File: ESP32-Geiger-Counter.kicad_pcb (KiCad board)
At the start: 2 copper layers, 137 x 104 mm, 85 parts, among them J1 2s1p Lipo Battery Pack (8.4V-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, J2 USB_C_Receptacle_USB2.0_16P, J5 Conn_01x07, Q1 STN1HNK60, Q3 2N7002, Q4 AO3401A, Q5 MMBT3904, SW1 SW_SPDT, SW2 RESET, SW3 BOOT, U1 BQ25886RGE, U2 AP63203WU, U3 ESP32-S3-WROOM-1, U4 UCC27517DBVR, U5 USBLC6-2SC6, U6 SBM-20 Geiger Mueller Tube

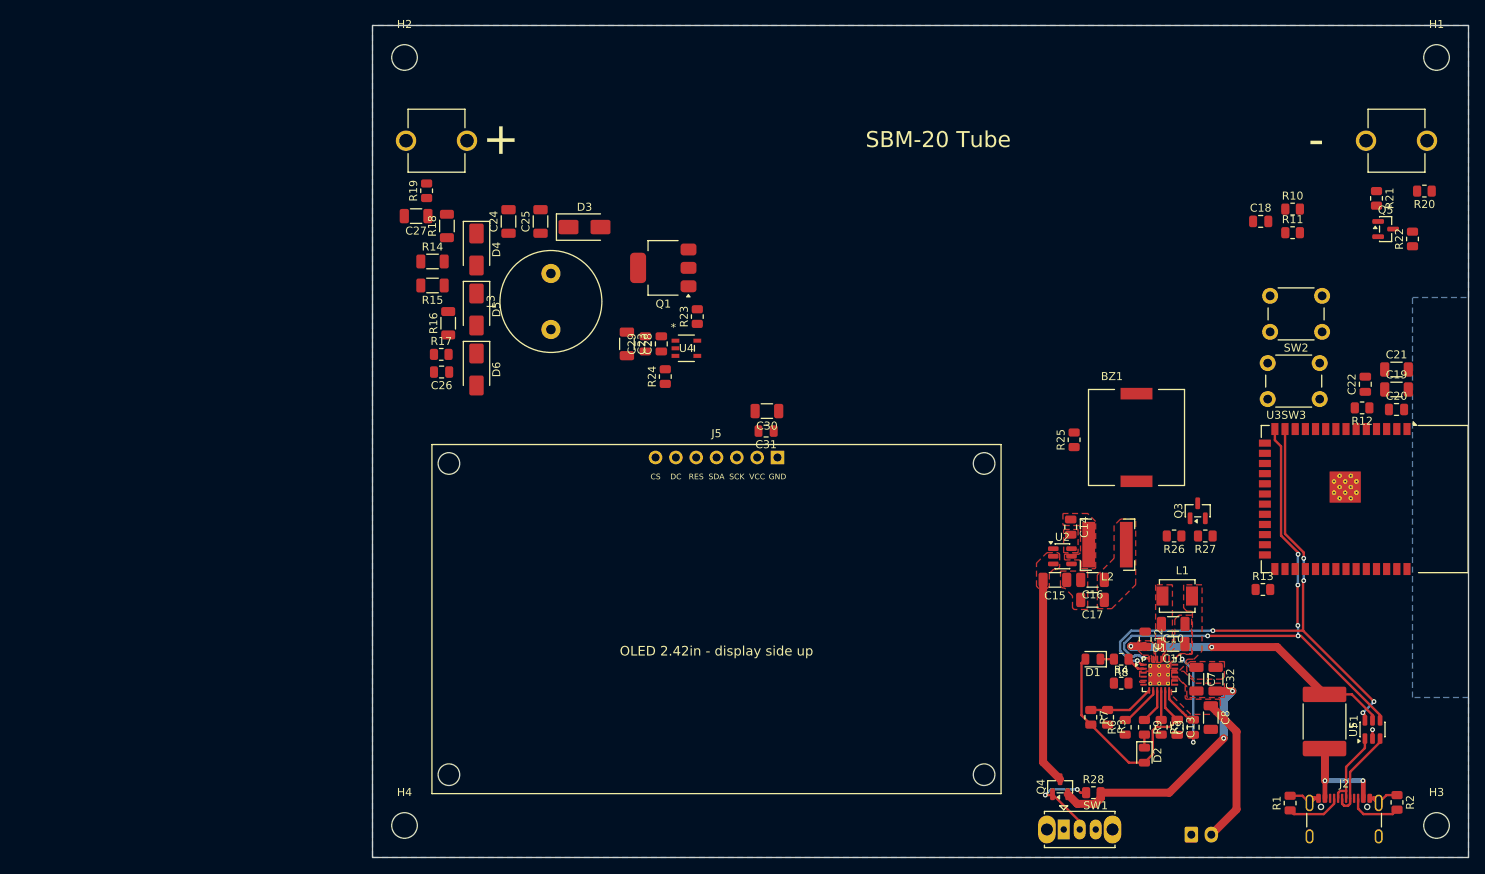
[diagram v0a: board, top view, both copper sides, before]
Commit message: layout stuff
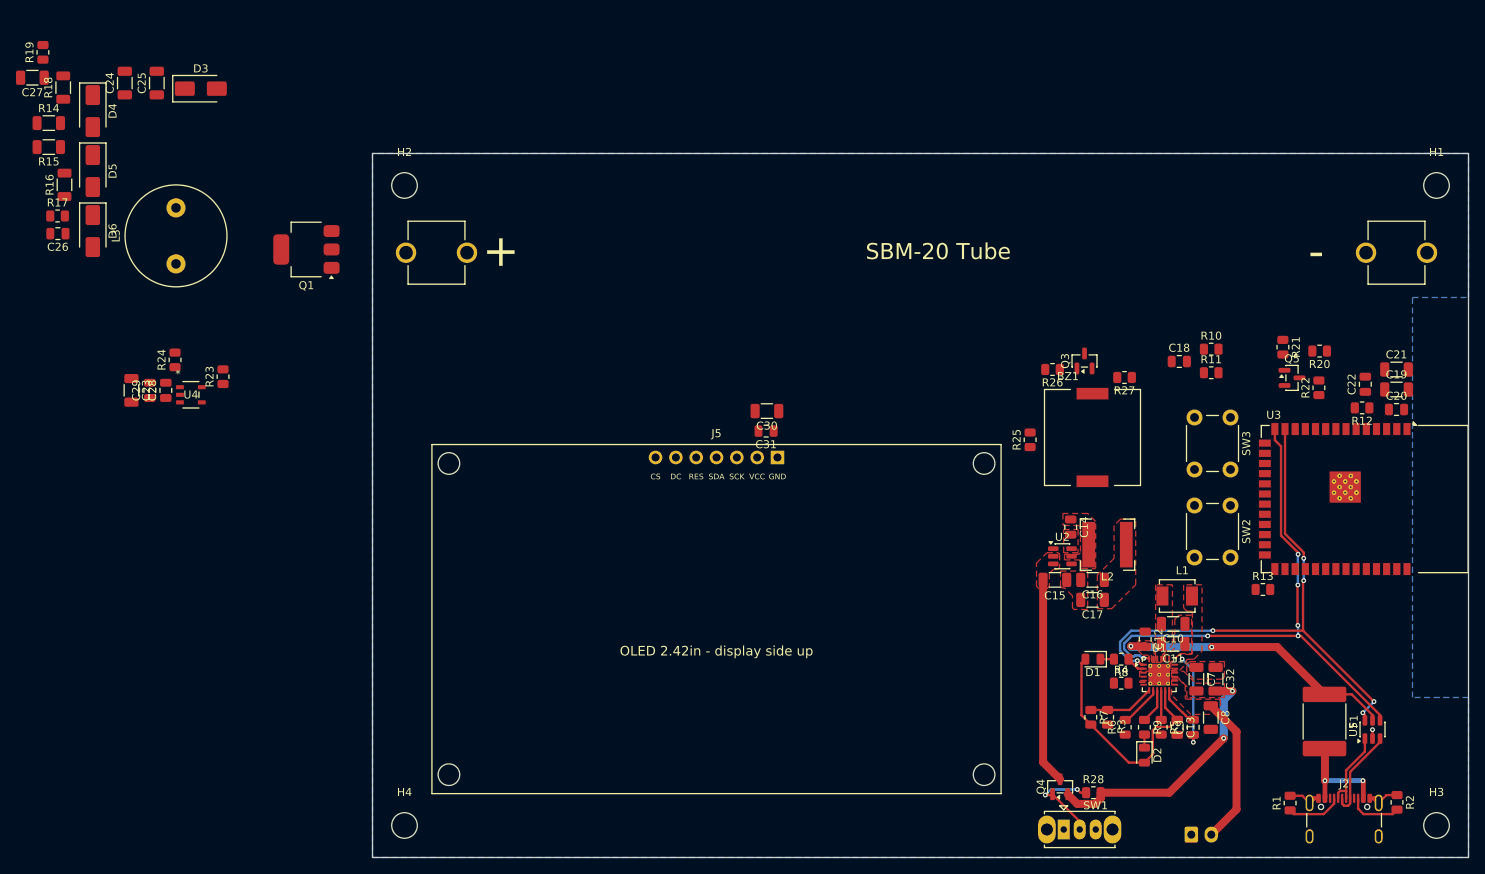
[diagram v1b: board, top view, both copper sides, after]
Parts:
- moved C23 62.2 mm to (66.9, 246.6)
- moved C28 62.2 mm to (71.2, 246.6)
- moved C29 62.2 mm to (69.2, 246.6)
- moved U4 62.2 mm to (74.3, 247.2)
- moved R24 61.3 mm to (72.3, 242.8)
- moved R23 59.8 mm to (78.3, 244.9)
- moved D4 51.0 mm to (62.0, 211.7)
- moved D5 51.0 mm to (62.0, 219.2)
- moved D6 51.0 mm to (62.0, 226.7)
- moved R14 51.0 mm to (56.5, 213.2)
- moved R15 51.0 mm to (56.5, 216.2)
- moved R16 51.0 mm to (58.5, 220.9)
- moved R18 51.0 mm to (58.3, 208.8)
- moved C24 51.0 mm to (66.0, 208.2)
- moved C25 51.0 mm to (70.0, 208.2)
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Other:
- board size 137 x 104 mm -> 137 x 88 mm
